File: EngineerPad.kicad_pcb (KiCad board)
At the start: 2 copper layers, 114.9 x 97.8 mm, 69 parts, among them J1 AVR ISP, J2 USB_A, SW1 SW_Push, SW10 SW_Push, SW11 SW_Push, SW12 SW_Push, SW13 SW_Push, SW14 SW_Push, SW15 SW_Push, SW16 SW_Push, SW17 SW_Push, SW18 SW_Push, SW19 SW_Push, SW2 SW_Push, SW20 SW_Push, SW21 SW_Push, SW22 SW_Push, SW23 SW_Push, SW3 SW_Push, SW4 SW_Push, SW5 SW_Push, SW6 SW_Push, SW7 SW_Push, SW8 SW_Push, SW9 SW_Push, U1 ATmega328P-PU, Y1 16MHz

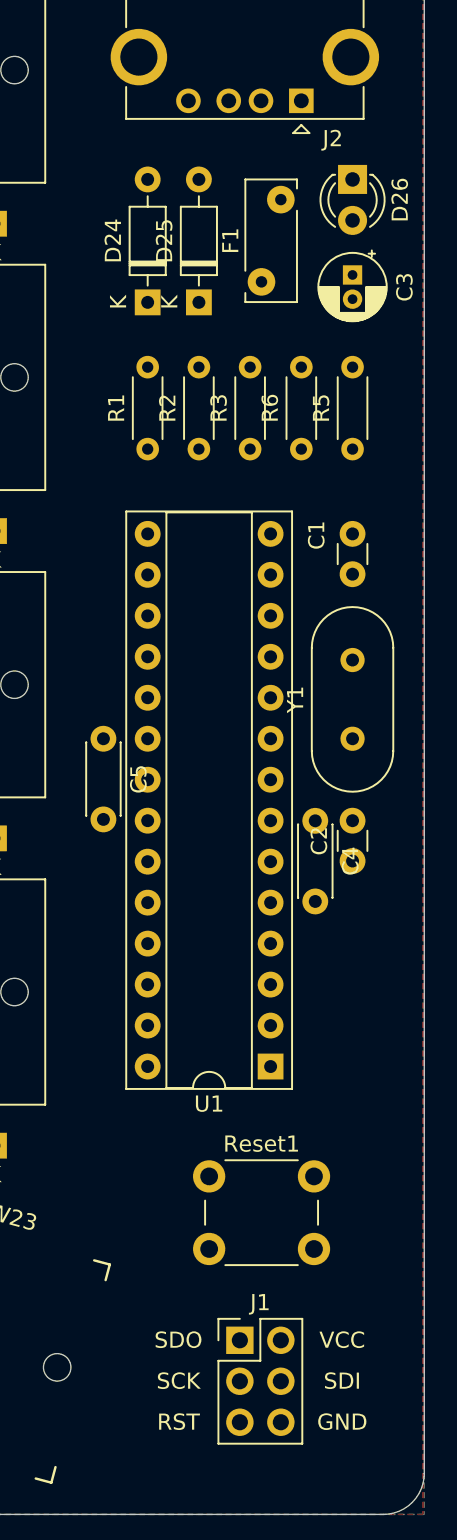
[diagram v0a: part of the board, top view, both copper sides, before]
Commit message: wip
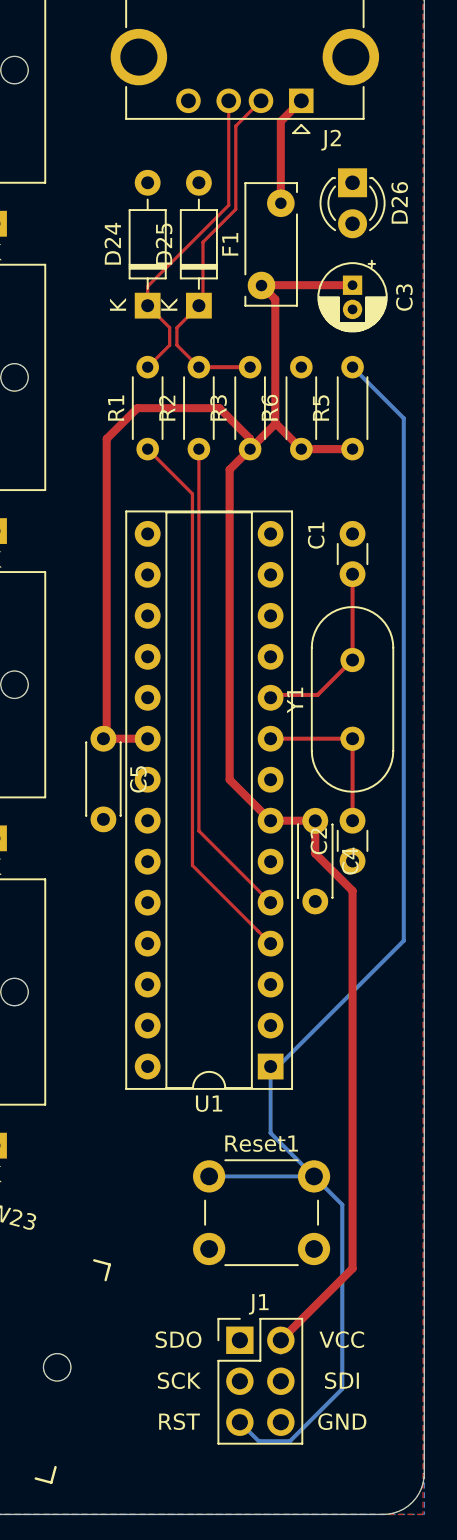
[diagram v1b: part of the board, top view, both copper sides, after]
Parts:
- moved C3 0.63 mm to (187.5, 79.8)
- moved F1 0.23 mm to (181.9, 79.9)
- moved D24 0.21 mm to (174.8, 81.1)
- moved D25 0.21 mm to (178.0, 81.1)
- moved D26 0.21 mm to (187.5, 73.5)
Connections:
- J1 pad 1: Row1 -> Col1
- J1 pad 3: Row0 -> Col0
- J1 pad 4: Row2 -> Col2
- U1 pad 15: Row0 -> Col4
- U1 pad 16: Row1 -> Col3
- U1 pad 17: Row2 -> Col2
- U1 pad 18: Row3 -> Col1
- U1 pad 19: Row4 -> Col0
- U1 pad 23: Col4 -> Row0
- U1 pad 24: Col3 -> Row1
- U1 pad 25: Col2 -> Row2
- U1 pad 26: Col1 -> Row3
- U1 pad 27: Col0 -> Row4
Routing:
- net +5V: track 0.00 -> 117.9 mm
- net Reset: track 0.00 -> 84.9 mm
- net D+: track 0.00 -> 33.8 mm
- net D-: track 0.00 -> 30.0 mm
- net /DN: track 0.00 -> 22.4 mm
- net /DP: track 0.00 -> 19.7 mm
- net Net-(C1-Pad2): track 0.00 -> 11.4 mm
- net Net-(C2-Pad2): track 0.00 -> 10.2 mm
- net Net-(F1-Pad2): track 0.00 -> 6.88 mm
